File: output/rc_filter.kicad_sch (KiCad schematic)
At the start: 2 parts

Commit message: feat: add capacitor, GND & Resistor symbols
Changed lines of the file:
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@@
-(kicad_sch (version 20230121) (generator icelang)
+(kicad_sch
+  (version 20240101)
+  (generator "icelang")
+  (generator_version "1.0")
   (paper "A4")
   (title_block (title "rc_filter"))
   (symbol
     (lib_id "Device:R")
-    (at -15.24 5.08 0)
+    (at 150.0 87.3 90)
     (unit 1)
-    (in_bom yes) (on_board yes)
-    (property "Reference" "R1" (at -15.24 3.58 0) (effects (font (size 1.27 1.27))))
-    (property "Value" "10k" (at -15.24 6.58 0) (effects (font (size 1.27 1.27))))
+    (in_bom yes)
+    (on_board yes)
+    (property "Reference" "R1"
+      (at 152.032 87.3 90)
+      (effects (font (size 1.27 1.27)))
+    )
+    (property "Value" "10k"
+      (at 147.968 87.3 90)
+      (effects (font (size 1.27 1.27)))
+    )
+    (property "Footprint" "" (at 0 0 0)
+      (effects (font (size 1.27 1.27)) hide)
+    )
+    (property "Datasheet" "~" (at 0 0 0)
+      (effects (font (size 1.27 1.27)) hide)
+    )
+    (instances
+      (project "schematic"
+        (path "/e9ca51da-7e16-4b28-a990-e408861a3db7"
+          (reference "R1")
+          (unit 1)
+        )
+      )
+    )
   )
   (symbol
     (lib_id "Device:C")
-    (at 15.24 0.0 0)
+    (at 188.1 138.1 90)
     (unit 1)
-    (in_bom yes) (on_board yes)
-    (property "Reference" "C1" (at 15.24 -1.5 0) (effects (font (size 1.27 1.27))))
-    (property "Value" "10F" (at 15.24 1.5 0) (effects (font (size 1.27 1.27))))
+    (in_bom yes)
+    (on_board yes)
+    (property "Reference" "C1"
+      (at 190.132 138.1 90)
+      (effects (font (size 1.27 1.27)))
+    )
+    (property "Value" "10F"
+      (at 186.068 138.1 90)
+      (effects (font (size 1.27 1.27)))
+    )
+    (property "Footprint" "" (at 0 0 0)
+      (effects (font (size 1.27 1.27)) hide)
+    )
+    (property "Datasheet" "~" (at 0 0 0)
+      (effects (font (size 1.27 1.27)) hide)
+    )
+    (instances
+      (project "schematic"
+        (path "/e9ca51da-7e16-4b28-a990-e408861a3db7"
+          (reference "C1")
+          (unit 1)
+        )
+      )
+    )
   )
   (symbol
     (lib_id "power:GND")
-    (at 0.0 -15.24 0)
+    (at 150.0 176.2 0)
     (unit 1)
-    (in_bom yes) (on_board yes)
-    (property "Reference" "#PWR" (at 0.0 -15.24 0) (effects (font (size 1.27 1.27)) hide))
-    (property "Value" "GND" (at 0.0 -16.740000000000002 0) (effects (font (size 1.27 1.27))))
+    (in_bom yes)
+    (on_board yes)
+    (property "Reference" "#PWR01"
+      (at 150.0 178.2 0)
+      (effects (font (size 1.27 1.27)) hide)
+    )
+    (property "Value" "GND"
+      (at 150.0 179.7 0)
+      (effects (font (size 1.27 1.27)))
+    )
+    (property "Footprint" "" (at 0 0 0)
+      (effects (font (size 1.27 1.27)) hide)
+    )
+    (property "Datasheet" "" (at 0 0 0)
+      (effects (font (size 1.27 1.27)) hide)
+    )
+    (instances
+      (project "schematic"
+        (path "/e9ca51da-7e16-4b28-a990-e408861a3db7"
+          (reference "#PWR01")
+          (unit 1)
+        )
+      )
+    )
+  )
+  (global_label "VIN"
+    (shape input)
+    (at 73.8 74.6 0)
+    (fields_autoplaced yes)
+    (effects (font (size 1.27 1.27)))
+    (property "Intersheet References" "${INTERSHEET_REFS}"
+      (at 0 0 0)
+      (effects (font (size 1.27 1.27)) hide)
+    )
+  )
+  (global_label "VOUT"
+    (shape output)
+    (at 226.2 100.0 0)
+    (fields_autoplaced yes)
+    (effects (font (size 1.27 1.27)))
+    (property "Intersheet References" "${INTERSHEET_REFS}"
+      (at 0 0 0)
+      (effects (font (size 1.27 1.27)) hide)
+    )
   )
   (wire
-    (pts (xy -15.2 5.1) (xy -15.2 0.0))
+    (pts (xy 74.0 74.5) (xy 74.0 100.0))
     (stroke (width 0) (type default))
   )
   (wire
-    (pts (xy -15.2 0.0) (xy 15.2 0.0))
+    (pts (xy 74.0 100.0) (xy 226.0 100.0))
     (stroke (width 0) (type default))
   )
   (wire
-    (pts (xy 15.2 0.0) (xy 15.2 -0.1))
+    (pts (xy 226.0 100.0) (xy 226.0 100.5))
     (stroke (width 0) (type default))
   )
   (wire
-    (pts (xy 15.2 -0.1) (xy 0.0 -0.1))
+    (pts (xy 226.0 100.5) (xy 150.0 100.5))
     (stroke (width 0) (type default))
   )
   (wire
-    (pts (xy 0.0 -0.1) (xy 0.0 -15.2))
+    (pts (xy 150.0 100.5) (xy 150.0 176.0))
     (stroke (width 0) (type default))
   )
+  (sheet_instances
+    (path "/"
+      (page "1")
+    )
+  )
 )

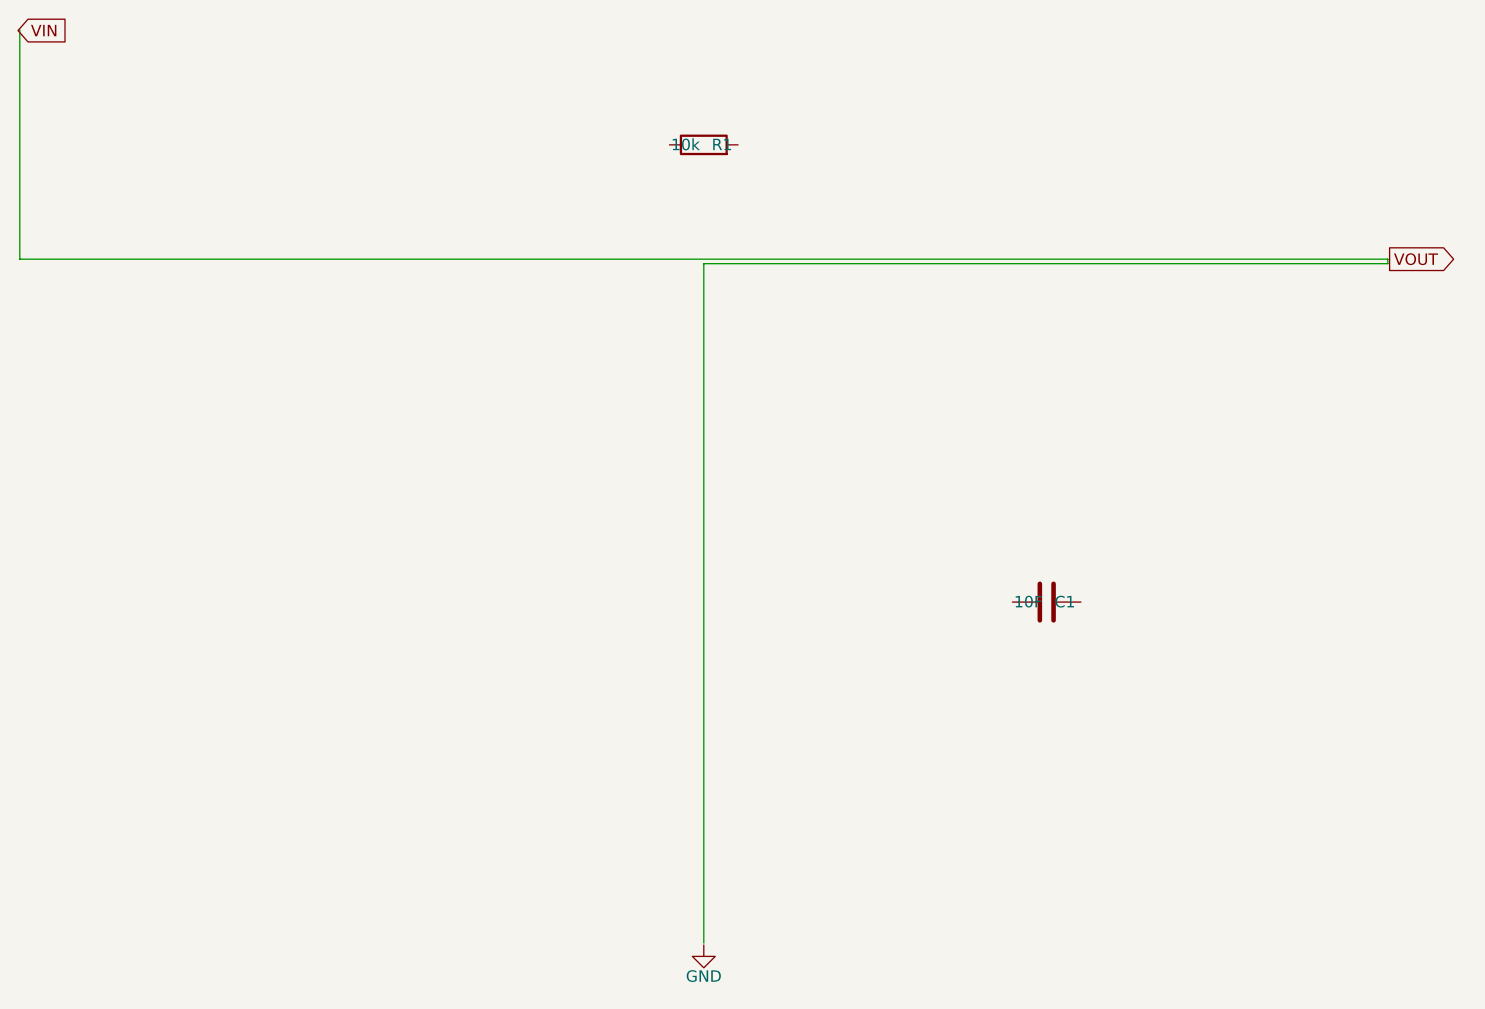
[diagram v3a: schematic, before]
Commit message: feat: the core pipelines works
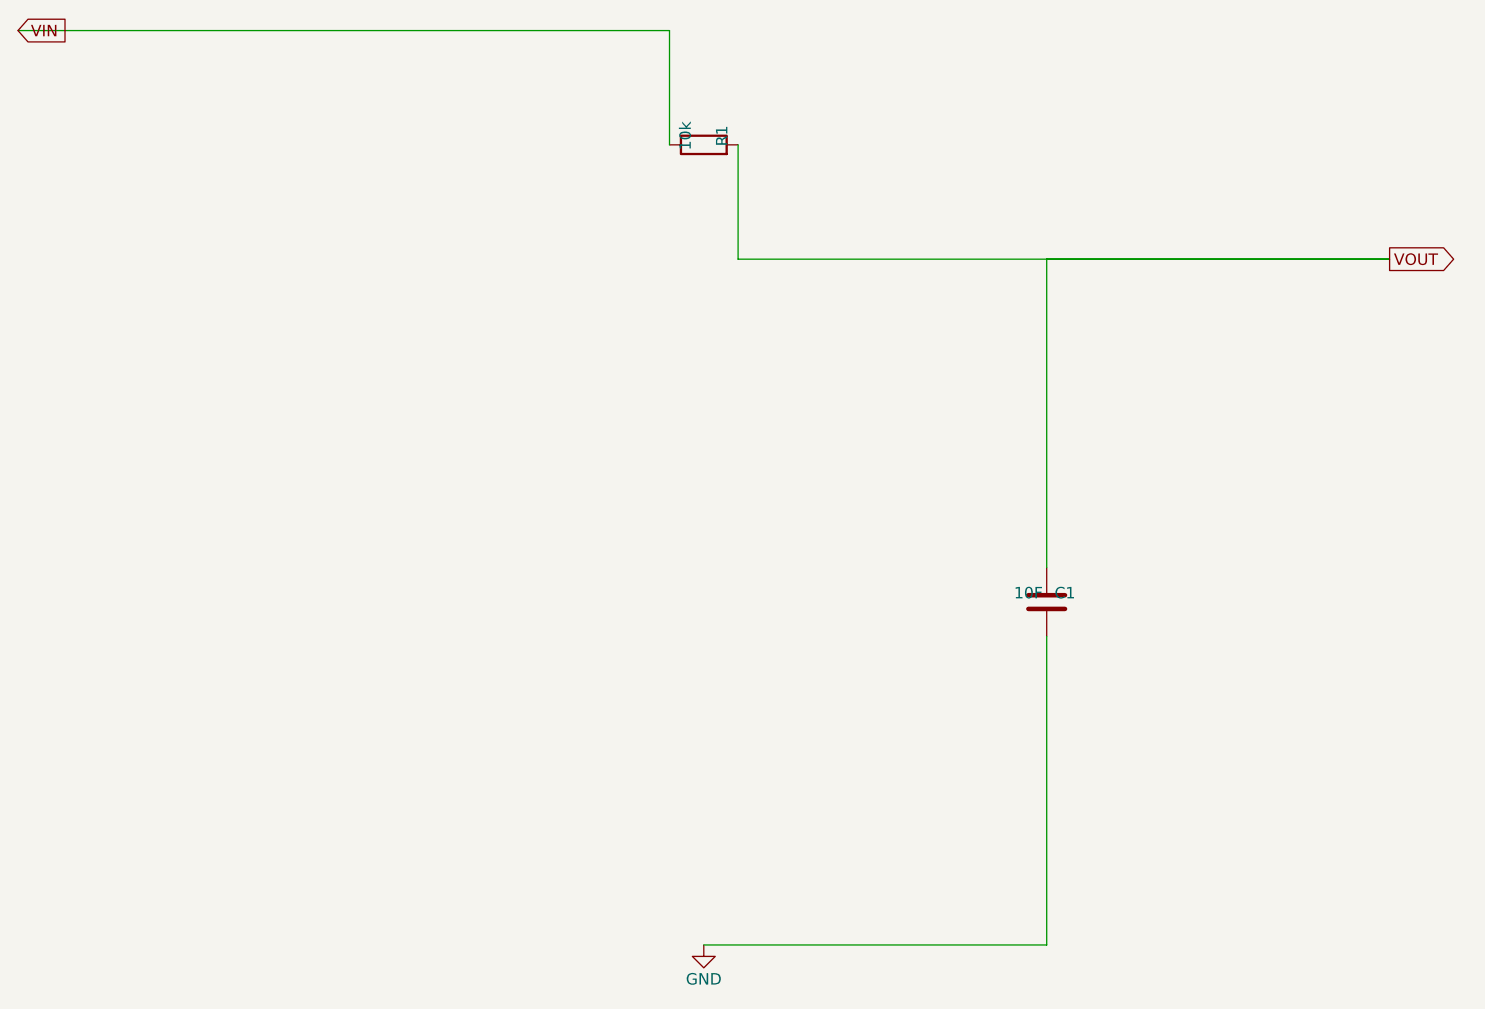
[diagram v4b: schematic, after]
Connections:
- net GND: now also C1.2
- net VIN: now also R1.1
- net VOUT: now also C1.1, R1.2
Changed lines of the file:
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@@
     (on_board yes)
     (property "Reference" "R1"
-      (at 152.032 87.3 90)
+      (at 152.032 86.3 0)
       (effects (font (size 1.27 1.27)))
     )
     (property "Value" "10k"
-      (at 147.968 87.3 90)
+      (at 147.968 86.3 0)
       (effects (font (size 1.27 1.27)))
     )
@@
     (instances
       (project "schematic"
-        (path "/38c0b97d-882d-4522-b078-8a3e8be254eb"
+        (path "/9c60ce1c-633a-4e5d-81ca-ae624066156c"
           (reference "R1")
           (unit 1)
@@
   (symbol
     (lib_id "Device:C")
-    (at 188.1 138.1 90)
+    (at 188.1 138.1 0)
     (unit 1)
     (in_bom yes)
     (on_board yes)
     (property "Reference" "C1"
-      (at 190.132 138.1 90)
+      (at 190.132 137.1 0)
       (effects (font (size 1.27 1.27)))
     )
     (property "Value" "10F"
-      (at 186.068 138.1 90)
+      (at 186.068 137.1 0)
       (effects (font (size 1.27 1.27)))
     )
@@
     (instances
       (project "schematic"
-        (path "/38c0b97d-882d-4522-b078-8a3e8be254eb"
+        (path "/9c60ce1c-633a-4e5d-81ca-ae624066156c"
           (reference "C1")
           (unit 1)
@@
     (on_board yes)
     (property "Reference" "#PWR01"
-      (at 150.0 178.2 0)
+      (at 150.0 182.55 0)
       (effects (font (size 1.27 1.27)) hide)
     )
     (property "Value" "GND"
-      (at 150.0 179.7 0)
+      (at 150.0 180.01 0)
       (effects (font (size 1.27 1.27)))
     )
@@
     (instances
       (project "schematic"
-        (path "/38c0b97d-882d-4522-b078-8a3e8be254eb"
+        (path "/9c60ce1c-633a-4e5d-81ca-ae624066156c"
           (reference "#PWR01")
           (unit 1)
@@
   )
   (wire
-    (pts (xy 74.0 74.5) (xy 74.0 100.0))
+    (pts (xy 73.8 74.6) (xy 146.19 74.6))
     (stroke (width 0) (type default))
   )
   (wire
-    (pts (xy 74.0 100.0) (xy 226.0 100.0))
+    (pts (xy 146.19 74.6) (xy 146.19 87.3))
     (stroke (width 0) (type default))
   )
   (wire
-    (pts (xy 226.0 100.0) (xy 226.0 100.5))
+    (pts (xy 226.2 100.0) (xy 153.81 100.0))
     (stroke (width 0) (type default))
   )
   (wire
-    (pts (xy 226.0 100.5) (xy 150.0 100.5))
+    (pts (xy 153.81 100.0) (xy 153.81 87.3))
     (stroke (width 0) (type default))
   )
   (wire
-    (pts (xy 150.0 100.5) (xy 150.0 176.0))
+    (pts (xy 226.2 100.0) (xy 188.1 100.0))
     (stroke (width 0) (type default))
   )
+  (wire
+    (pts (xy 188.1 100.0) (xy 188.1 134.29))
+    (stroke (width 0) (type default))
+  )
+  (wire
+    (pts (xy 150.0 176.2) (xy 188.1 176.2))
+    (stroke (width 0) (type default))
+  )
+  (wire
+    (pts (xy 188.1 176.2) (xy 188.1 141.91))
+    (stroke (width 0) (type default))
+  )
